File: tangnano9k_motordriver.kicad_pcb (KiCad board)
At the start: 2 copper layers, 115.6 x 92.7 mm, 30 parts, among them J1 Jack-DC, J2 Screw_Terminal_01x04, J3 Screw_Terminal_01x04, J4 Reserve, J5 Reserve, J6 Reserve, J7 Reserve_PinHeader, J8 Pmod, SW3 SW_DIP_x08, U1 BP5293-5, U2 TB67S101ANG, U3 TangNano9K, U4 OSL641505-BB, U5 TB67S101ANG

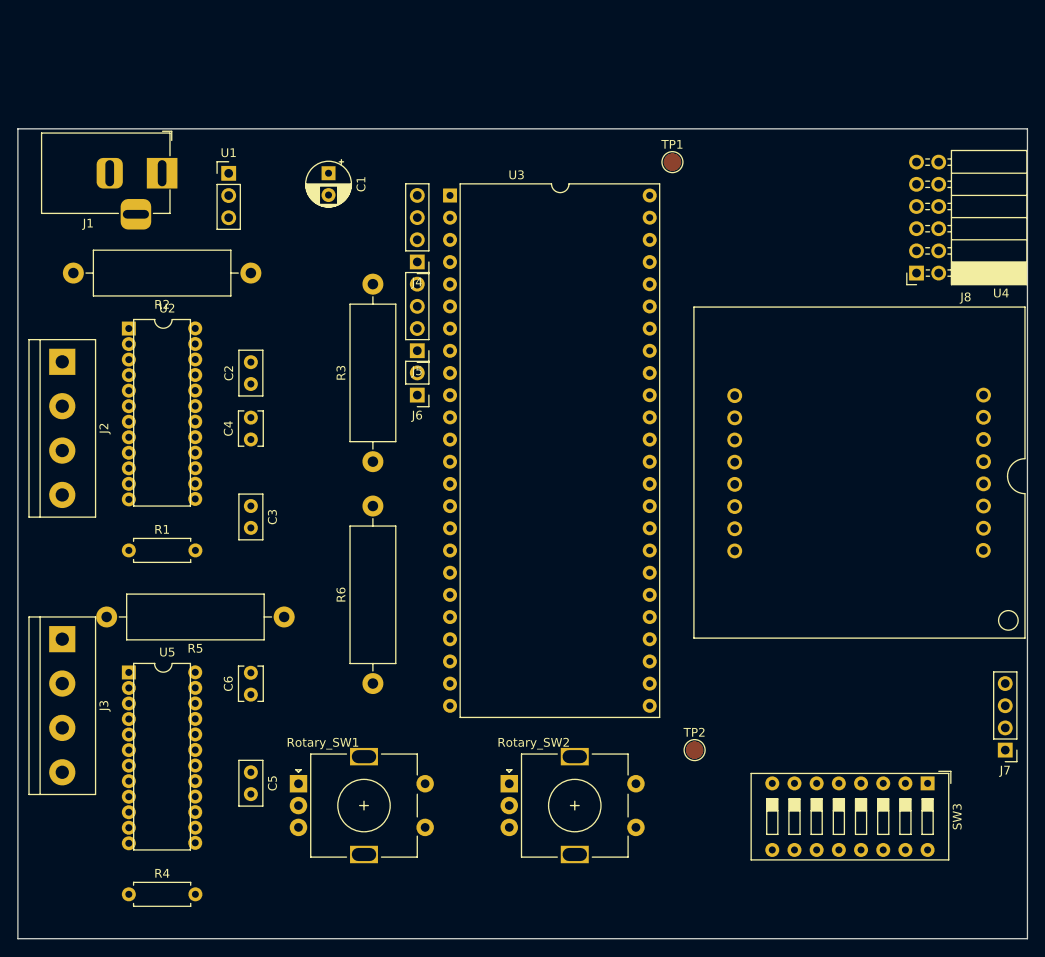
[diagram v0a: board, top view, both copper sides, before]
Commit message: 7
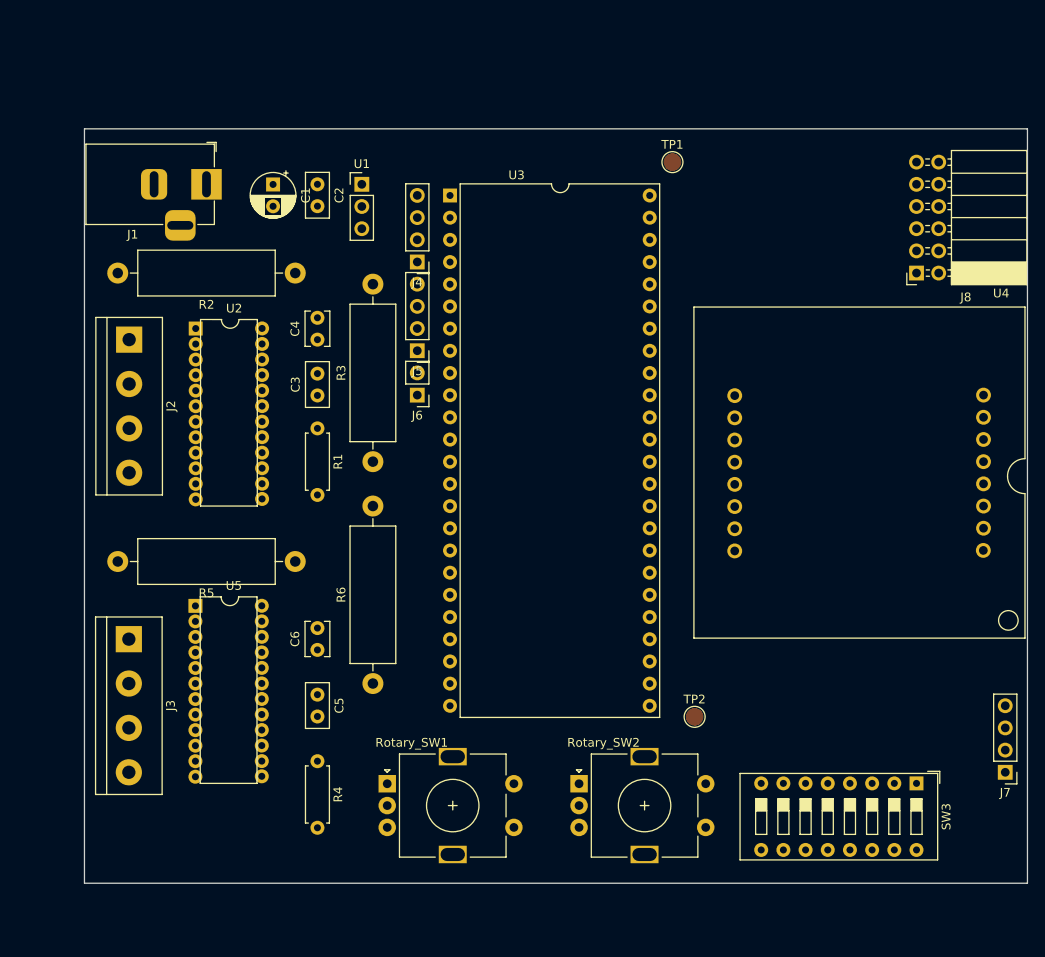
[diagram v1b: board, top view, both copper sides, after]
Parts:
- moved R4 26.4 mm to (86.4, 132.1), turned to -90 degrees
- moved R1 25.7 mm to (86.4, 94.0), turned to -90 degrees
- moved C2 24.1 mm to (86.4, 66.0), turned to -90 degrees
- moved U1 15.3 mm to (91.4, 66.0)
- moved C3 14.8 mm to (86.4, 90.2), turned to 90 degrees
- moved C4 13.7 mm to (86.4, 83.8)
- moved C5 11.7 mm to (86.4, 124.5)
- moved U5 10.8 mm to (72.4, 114.3)
- moved Rotary_SW1 10.2 mm to (94.3, 134.7)
- moved C6 9.18 mm to (86.4, 119.3)
- moved J2 8.07 mm to (64.8, 83.8)
- moved Rotary_SW2 7.99 mm to (116.3, 134.7)
- moved U2 7.66 mm to (72.4, 82.5)
- moved J3 7.62 mm to (64.8, 118.1)
- moved C1 6.48 mm to (81.3, 66.1)
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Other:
- board size 115.6 x 92.7 mm -> 107.9 x 86.4 mm

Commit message: 8
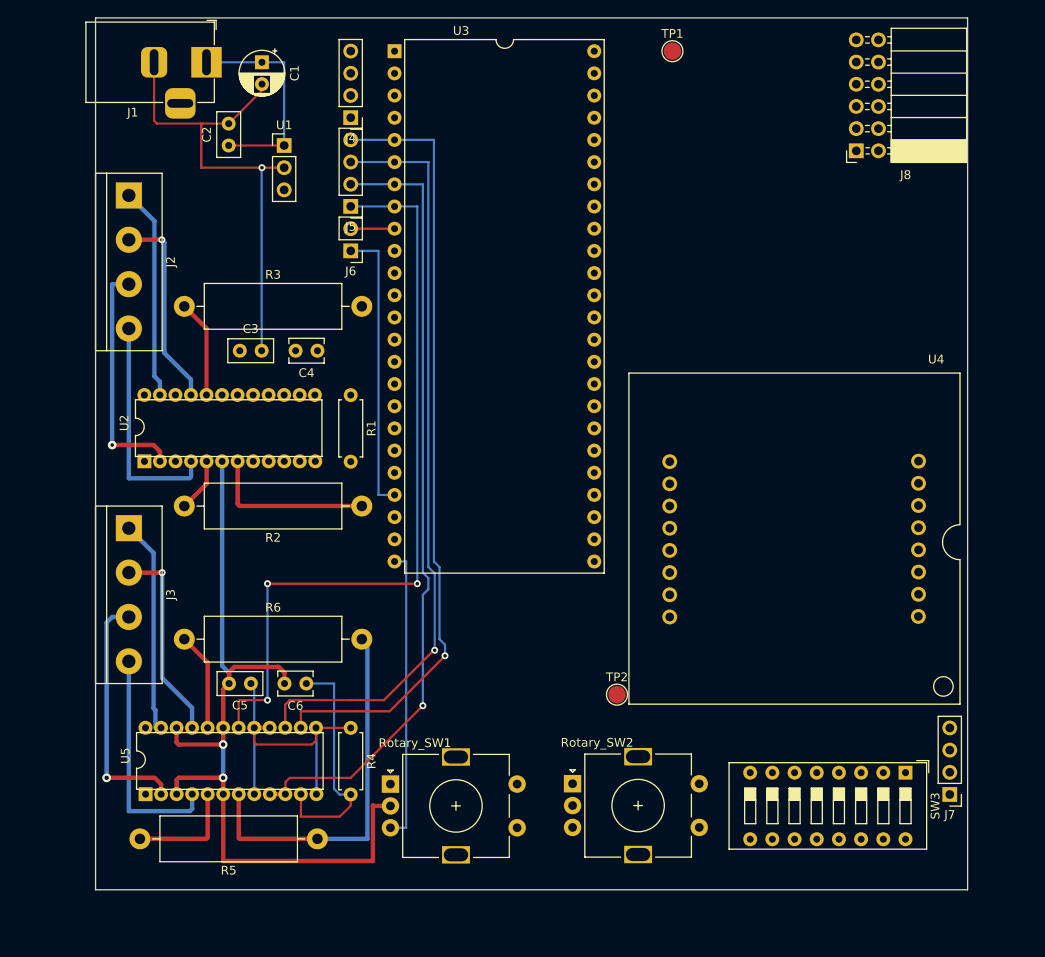
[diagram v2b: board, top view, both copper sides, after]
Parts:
- moved R5 31.9 mm to (86.4, 141.0)
- moved R3 28.0 mm to (71.1, 80.0), turned to 0 degrees
- moved R2 27.7 mm to (91.4, 102.9)
- moved U5 22.3 mm to (66.7, 135.9), turned to 90 degrees
- moved R6 22.2 mm to (71.1, 118.1), turned to 0 degrees
- moved J4 18.2 mm to (90.2, 58.4)
- moved J5 18.2 mm to (90.2, 68.6)
- moved J6 18.2 mm to (90.2, 73.7)
- moved U3 17.7 mm to (95.2, 50.8)
- moved J2 16.5 mm to (64.8, 67.3)
- moved U2 16.3 mm to (66.6, 97.8), turned to 90 degrees
- moved J8 15.6 mm to (148.0, 62.2)
- moved C1 14.0 mm to (80.0, 52.1)
- moved J1 14.0 mm to (73.7, 52.1)
- moved J3 12.7 mm to (64.8, 105.4)
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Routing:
- net GND: track 0.00 -> 152.5 mm, vias 0 -> 3
- net /VREF_2: track 0.00 -> 91.0 mm, vias 0 -> 1
- net /PHASEA_2: track 0.00 -> 90.1 mm, vias 0 -> 1
- net /STANBY_2: track 0.00 -> 87.7 mm, vias 0 -> 3
- net /PHASEB_2: track 0.00 -> 87.4 mm, vias 0 -> 1
- net Net-(C1-Pad1): track 0.00 -> 86.8 mm
- net Net-(C5-Pad1): track 0.00 -> 36.7 mm
- net /B_1: track 0.00 -> 33.6 mm
- net Net-(J6-Pad1): track 0.00 -> 33.0 mm
- net Net-(J3-Pad3): track 0.00 -> 28.3 mm, vias 0 -> 1
- net Net-(C6-Pad1): track 0.00 -> 27.5 mm
- net Net-(J2-Pad3): track 0.00 -> 27.2 mm, vias 0 -> 1
- net Net-(J3-Pad4): track 0.00 -> 26.2 mm
- net Net-(J2-Pad4): track 0.00 -> 26.1 mm
- net Net-(J2-Pad1): track 0.00 -> 24.3 mm
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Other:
- board size 107.9 x 86.4 mm -> 99.8 x 99.8 mm
